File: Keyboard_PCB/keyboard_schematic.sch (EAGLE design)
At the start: 266 parts, among them IC1 LMV321M5, M2 KEYSWITCH-RGBSMDLED-ALPSMX-1U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, M3 KEYSWITCH-RGBSMDLED-ALPSMX-1U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, M4 KEYSWITCH-RGBSMDLED-ALPSMX-1U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, M5 KEYSWITCH-RGBSMDLED-ALPSMX-1U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, M6 KEYSWITCH-RGBSMDLED-ALPSMX-1U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, T1 BC846, Y2 CRYSTAL-GROUNDEDSMD-3.2X2.5

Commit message: Updated Schematics and boards
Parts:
- removed IC2: (no value), controller-micro_atmel_jd:AT90USB-QFN
- removed U$2: PCB_USB_CDS_1, USB_pcb_connectors:PCB_USB_CDS_1
- added IC3: (no value), controller-micro_atmel_jd:AT90USB-TQFP
- added J1: 1-2295018-2, 1-2295018-2:1-2295018-2
- T1: value BC846 -> (none); device transistor:BC846 -> transistor:-NPN-SOT23-EBC
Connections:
- removed net COL11: EQUAL2.P0, KP_9.P0, KP_ASTERISK.P0, KP_DASH.P0, NEXTSONG.P0, PAUSEPLAY.P0
- removed net ROW1.1: DF1.C, DF11.C, DF3.C, DF5.C, DF7.C, DF9.C, DM6.C, DNEXTSONG1.C, DPAUSE.C, DPAUSEPLAY.C, DSCROLLLOCK.C, DVOLUMEUP.C
- removed net ROW1.2: DBACKSONG.C, DESC.C, DF10.C, DF12.C, DF2.C, DF4.C, DF6.C, DF8.C, DLOCK.C, DNEXTSONG.C, DPRTSC.C, DVOLUMNEDOWN.C
- removed net ROW2.1: D1.C, D3.C, D5.C, D7.C, D9.C, DBACKSPACE.C, DDASH.C, DHOME.C, DKP_DASH.C, DKP_SLASH.C, DM5.C
- removed net ROW2.2: D0.C, D2.C, D4.C, D6.C, D8.C, DEQUAL.C, DGRAVE.C, DINSERT.C, DKP_ASTERISK.C, DNUMLOCK.C, DPGUP.C, DUNDERSCORE.C
- removed net ROW3.1: DBACKSLASH.C, DE.C, DEND.C, DEQUAL2.C, DKP_8.C, DLBRACKET.C, DM4.C, DO.C, DQ.C, DT.C, DU.C
- removed net ROW3.2: DDELETE.C, DI.C, DKP_5.C, DKP_7.C, DKP_9.C, DP.C, DPGDN.C, DR.C, DRBRACKET.C, DTAB.C, DW.C, DY.C
- removed net ROW4.1: DA.C, DCTRL2.C, DD.C, DG.C, DJ.C, DKP_4.C, DKP_6.C, DKP_62.C, DL.C, DM3.C, DQUOTE.C
- removed net ROW4.2: DCAPSLOCK.C, DENTER.C, DENTER2.C, DF.C, DH.C, DK.C, DKP_52.C, DS.C, DSEMICOLON.C, DUP.C
- removed net ROW5.1: DB.C, DC.C, DKP_2.C, DLEFT.C, DM.C, DM2.C, DMENU.C, DPERIOD.C, DZ.C
- removed net ROW5.2: DCOMMA.C, DDELETE2.C, DKP_1.C, DKP_3.C, DN.C, DRIGHT.C, DSHIFT.C, DSHIFT2.C, DSLASH.C, DV.C, DX.C
- removed net ROW6.1: DALT.C, DALT2.C, DBACKSPACE_1.C, DCTRL.C, DDOWN.C, DKP_0.C, DKP_DEL.C, DM1.C, DSPACE.C, DWIN.C, DWIN2.C
- new net COL13: 0.P0, F10.P0, P.P0, SEMICOLON.P0, SLASH.P0, WIN2.P0
- new net COL14: DASH.P0, F11.P0, LBRACKET.P0, MENU.P0, QUOTE.P0
- new net COL15: EQUAL.P0, F12.P0, RBRACKET.P0
- new net COL16: VOLUMEUP.P0
- new net COL17: BACKSLASH.P0, BACKSPACE.P0, CTRL2.P0, ENTER.P0, SHIFT2.P0, VOLUMNEDOWN.P0
- new net COL18: DELETE.P0, INSERT.P0, LEFT.P0, PRTSC.P0
- new net COL19: DOWN.P0, END.P0, HOME.P0, SCROLLLOCK.P0, UP.P0
- new net COL20: PAUSE.P0, PGDN.P0, PGUP.P0, RIGHT.P0
- new net COL21: BACKSONG.P0, KP_0.P0, KP_1.P0, KP_4.P0, KP_7.P0, NUMLOCK.P0
- new net COL22: KP_2.P0, KP_52.P0, KP_8.P0, KP_SLASH.P0, PAUSEPLAY.P0
- new net COL23: KP_3.P0, KP_6.P0, KP_9.P0, KP_ASTERISK.P0, KP_DEL.P0, NEXTSONG.P0
- new net COL24: ENTER2.P0, EQUAL2.P0, KP_DASH.P0, RANDSONG.P0
- new net COL25: BACKSPACE_1.P0, KP_5.P0, KP_62.P0, KP_DELETE2.P0, LOCK.P0, UNDERSCORE.P0
- new net LED1: M6.DI
- new net LED2: M5.DI
- new net LED3: M4.DI
- new net LED4: M3.DI
- new net LED5: M2.DI
- new net LED6: CTRL1.DI
- new net N$107: ESC.DI, M6.DO
- new net N$118: ESC.DO, F1.DI
- new net N$119: F1.DO, F2.DI
- new net N$121: F2.DO, F3.DI
- new net N$122: F3.DO, F4.DI
- new net N$123: F4.DO, F5.DI
- new net N$124: F5.DO, F6.DI
- new net N$132: F6.DO, F7.DI
- new net N$133: F7.DO, F8.DI
- new net N$134: F8.DO, F9.DI
- new net N$135: F10.DI, F9.DO
- new net N$136: F10.DO, F11.DI
- new net N$137: F11.DO, F12.DI
- new net N$138: F12.DO, VOLUMEUP.DI
- new net N$139: VOLUMEUP.DO, VOLUMNEDOWN.DI
- new net N$140: PRTSC.DI, VOLUMNEDOWN.DO
- new net N$141: PRTSC.DO, SCROLLLOCK.DI
- new net N$142: PAUSE.DI, SCROLLLOCK.DO
- new net N$143: BACKSONG.DI, PAUSE.DO
- new net N$144: BACKSONG.DO, PAUSEPLAY.DI
- new net N$145: NEXTSONG.DI, PAUSEPLAY.DO
- new net N$146: NEXTSONG.DO, RANDSONG.DI
- new net N$147: LOCK.DI, RANDSONG.DO
- new net N$148: IC3.PA1_AD1
- new net N$149: GRAVE.DI, M5.DO
- new net N$150: 1.DI, GRAVE.DO
- new net N$151: 1.DO, 2.DI
- new net N$152: 2.DO, 3.DI
- new net N$153: 3.DO, 4.DI
- new net N$154: 4.DO, 5.DI
- new net N$155: 5.DO, 6.DI
- new net N$156: 6.DO, 7.DI
- new net N$157: 7.DO, 8.DI
- new net N$158: 8.DO, 9.DI
- new net N$159: 0.DI, 9.DO
- new net N$160: 0.DO, DASH.DI
- new net N$161: DASH.DO, EQUAL.DI
- new net N$162: IC3.PA2_AD2
- new net N$163: BACKSPACE.DI, EQUAL.DO
- new net N$164: BACKSPACE.DO, INSERT.DI
- new net N$165: HOME.DI, INSERT.DO
- new net N$166: HOME.DO, PGUP.DI
- new net N$167: NUMLOCK.DI, PGUP.DO
- new net N$168: KP_SLASH.DI, NUMLOCK.DO
- new net N$169: KP_ASTERISK.DI, KP_SLASH.DO
- new net N$170: KP_ASTERISK.DO, KP_DASH.DI
- new net N$171: KP_DASH.DO, UNDERSCORE.DI
- new net N$172: M4.DO, TAB.DI
- new net N$173: Q.DI, TAB.DO
- new net N$174: Q.DO, W.DI
- new net N$175: E.DI, W.DO
- new net N$176: E.DO, R.DI
- new net N$177: R.DO, T.DI
- new net N$178: T.DO, Y.DI
- new net N$179: U.DI, Y.DO
- new net N$180: I.DI, U.DO
- new net N$181: I.DO, O.DI
- new net N$182: O.DO, P.DI
- new net N$183: LBRACKET.DI, P.DO
- new net N$184: LBRACKET.DO, RBRACKET.DI
- new net N$185: BACKSLASH.DI, RBRACKET.DO
- new net N$186: IC3.PA3_AD3
- new net N$187: BACKSLASH.DO, DELETE.DI
- new net N$188: DELETE.DO, END.DI
- new net N$189: END.DO, PGDN.DI
- new net N$190: KP_7.DI, PGDN.DO
- new net N$191: KP_7.DO, KP_8.DI
- new net N$192: KP_8.DO, KP_9.DI
- new net N$193: EQUAL2.DI, KP_9.DO
- new net N$194: EQUAL2.DO, KP_5.DI
- new net N$195: CAPSLOCK.DI, M3.DO
- new net N$196: A.DI, CAPSLOCK.DO
- new net N$197: A.DO, S.DI
- new net N$198: D.DI, S.DO
- new net N$199: D.DO, F.DI
- new net N$200: F.DO, G.DI
- new net N$201: G.DO, H.DI
- new net N$202: H.DO, J.DI
- new net N$203: J.DO, K.DI
- new net N$204: K.DO, L.DI
- new net N$205: L.DO, SEMICOLON.DI
- new net N$206: QUOTE.DI, SEMICOLON.DO
- new net N$207: ENTER.DI, QUOTE.DO
- new net N$208: ENTER.DO, KP_4.DI
- new net N$209: ENTER2.DI, KP_3.DO
- new net N$210: KP_4.DO, KP_52.DI
- new net N$211: KP_52.DO, KP_6.DI
- new net N$212: KP_6.DO, KP_62.DI
- new net N$213: IC3.PA4_AD4
- new net N$214: M2.DO, SHIFT.DI
- new net N$215: SHIFT.DO, Z.DI
- new net N$216: X.DI, Z.DO
- new net N$217: C.DI, X.DO
- new net N$218: C.DO, V.DI
- new net N$219: B.DI, V.DO
- new net N$220: B.DO, N.DI
- new net N$221: M.DI, N.DO
- new net N$222: COMMA.DI, M.DO
- new net N$223: COMMA.DO, PERIOD.DI
- new net N$224: PERIOD.DO, SLASH.DI
- new net N$225: SHIFT2.DI, SLASH.DO
- new net N$226: IC3.PA5_AD5
- new net N$227: KP_1.DO, KP_2.DI
- new net N$228: KP_2.DO, KP_3.DI
- new net N$229: ENTER2.DO, KP_DELETE2.DI
- new net N$230: KP_1.DI, SHIFT2.DO
- new net N$231: IC3.PA6_AD6
- new net N$232: CTRL.DI, CTRL1.DO
- new net N$233: CTRL.DO, WIN.DI
- new net N$234: ALT.DI, WIN.DO
- new net N$235: ALT.DO, SPACE.DI
- new net N$236: IC3.PA7_AD7
- new net N$238: ALT2.DI, SPACE.DO
- new net N$239: J1.VBUS@4
- new net N$242: ALT2.DO, WIN2.DI
- new net N$243: MENU.DI, WIN2.DO
- new net N$245: CTRL2.DI, MENU.DO
- new net N$246: CTRL2.DO, LEFT.DI
- new net N$247: KP_0.DI
- new net N$248: KP_0.DO, KP_DEL.DI
- new net N$249: BACKSPACE_1.DI, KP_DEL.DO
- new net N$250: DOWN.DI, LEFT.DO
- new net N$251: DOWN.DO, RIGHT.DI
- new net N$252: RIGHT.DO
- new net ROW1: DBACKSONG.C, DESC.C, DF1.C, DF10.C, DF11.C, DF12.C, DF2.C, DF3.C, DF4.C, DF5.C, DF6.C, DF7.C, DF8.C, DF9.C, DLOCK.C, DM6.C, DNEXTSONG.C, DNEXTSONG1.C, DPAUSE.C, DPAUSEPLAY.C, DPRTSC.C, DSCROLLLOCK.C, DVOLUMEUP.C, DVOLUMNEDOWN.C
- new net ROW2: D0.C, D1.C, D2.C, D3.C, D4.C, D5.C, D6.C, D7.C, D8.C, D9.C, DBACKSPACE.C, DDASH.C, DEQUAL.C, DGRAVE.C, DHOME.C, DINSERT.C, DKP_ASTERISK.C, DKP_DASH.C, DKP_SLASH.C, DM5.C, DNUMLOCK.C, DPGUP.C, DUNDERSCORE.C
- new net ROW3: DBACKSLASH.C, DDELETE.C, DE.C, DEND.C, DEQUAL2.C, DI.C, DKP_5.C, DKP_7.C, DKP_8.C, DKP_9.C, DLBRACKET.C, DM4.C, DO.C, DP.C, DPGDN.C, DQ.C, DR.C, DRBRACKET.C, DT.C, DTAB.C, DU.C, DW.C, DY.C
- new net ROW4: DA.C, DCAPSLOCK.C, DD.C, DENTER.C, DF.C, DG.C, DH.C, DJ.C, DK.C, DKP_4.C, DKP_52.C, DKP_6.C, DKP_62.C, DL.C, DM3.C, DQUOTE.C, DS.C, DSEMICOLON.C
- new net ROW5: DB.C, DC.C, DCOMMA.C, DDELETE2.C, DENTER2.C, DKP_1.C, DKP_2.C, DKP_3.C, DM.C, DM2.C, DN.C, DPERIOD.C, DSHIFT.C, DSHIFT2.C, DSLASH.C, DUP.C, DV.C, DX.C, DZ.C
- new net ROW6: DALT.C, DALT2.C, DBACKSPACE_1.C, DCTRL2.C, DDOWN.C, DKP_0.C, DKP_DEL.C, DLEFT.C, DM1.C, DMENU.C, DRIGHT.C, DSPACE.C, DWIN.C, DWIN2.C
- net +5V: now also IC3.AREF, IC3.AVCC, IC3.VCC, IC3.VCC@1, J1.VBUS@1, J1.VBUS@2, J1.VBUS@3; no longer IC2.AREF, IC2.AVCC, IC2.VCC, IC2.VCC@1, U$2.A4, U$2.A9, U$2.B4, U$2.B9
- net CC1: now also IC1.+IN, J1.CC1, R6.2; no longer R5.1, U$2.A5
- net CC2: now also J1.CC2, R5.1; no longer IC1.+IN, R6.2, U$2.B5
- net COL1: no longer CAPSLOCK.P0, ESC.P0, GRAVE.P0, SHIFT.P0, TAB.P0
- net COL10: now also 8.P0, COMMA.P0, F8.P0, I.P0, K.P0; no longer BACKSONG.P0, ENTER2.P0, KP_3.P0, KP_6.P0, KP_7.P0, KP_8.P0, KP_DEL.P0, KP_SLASH.P0, NUMLOCK.P0, PAUSE.P0
- net COL12: now also 9.P0, ALT2.P0, F9.P0, L.P0, O.P0, PERIOD.P0; no longer BACKSPACE_1.P0, KP_5.P0, KP_62.P0, KP_DELETE2.P0, LOCK.P0, RANDSONG.P0, UNDERSCORE.P0
- net COL2: now also CAPSLOCK.P0, ESC.P0, GRAVE.P0, SHIFT.P0, TAB.P0; no longer 1.P0, 2.P0, A.P0, F1.P0, F2.P0, Q.P0, S.P0, W.P0, X.P0, Z.P0
- net COL3: now also 1.P0, A.P0, F1.P0, Q.P0, Z.P0; no longer 3.P0, 4.P0, C.P0, D.P0, E.P0, F.P0, F3.P0, F4.P0, R.P0, V.P0
- net COL4: now also 2.P0, F2.P0, S.P0, W.P0, X.P0; no longer 5.P0, 6.P0, B.P0, F5.P0, F6.P0, G.P0, H.P0, N.P0, T.P0, Y.P0
- net COL5: now also 3.P0, C.P0, D.P0, E.P0, F3.P0; no longer 7.P0, 8.P0, COMMA.P0, F7.P0, F8.P0, I.P0, J.P0, K.P0, M.P0, SPACE.P0, U.P0
- net COL6: now also 4.P0, F.P0, F4.P0, R.P0, V.P0; no longer 0.P0, 9.P0, ALT2.P0, F10.P0, F9.P0, L.P0, O.P0, P.P0, PERIOD.P0, SEMICOLON.P0, SLASH.P0
- net COL7: now also 5.P0, B.P0, F5.P0, G.P0, SPACE.P0, T.P0; no longer DASH.P0, ENTER.P0, EQUAL.P0, F11.P0, F12.P0, LBRACKET.P0, MENU.P0, QUOTE.P0, RBRACKET.P0, SHIFT2.P0, WIN2.P0
- net COL8: now also 6.P0, F6.P0, H.P0, N.P0, Y.P0; no longer BACKSLASH.P0, BACKSPACE.P0, CTRL2.P0, DELETE.P0, DOWN.P0, INSERT.P0, LEFT.P0, RIGHT.P0, UP.P0, VOLUMEUP.P0, VOLUMNEDOWN.P0
- net COL9: now also 7.P0, F7.P0, J.P0, M.P0, U.P0; no longer END.P0, HOME.P0, KP_0.P0, KP_1.P0, KP_2.P0, KP_4.P0, KP_52.P0, PGDN.P0, PGUP.P0, PRTSC.P0, SCROLLLOCK.P0
- net D+32U: now also IC3.D+; no longer IC2.D+
- net D+USB: now also J1.D+@1; no longer U$2.A6
- net D-32U4: now also IC3.D-; no longer IC2.D-
- net D-USB: now also J1.D-@1; no longer U$2.A7
- net GND: now also IC3.AGND, IC3.GND, IC3.GND@1, IC3.UGND, J1.GND@1, J1.GND@2, J1.GND@3, J1.GND@4, J1.SHIELD; no longer IC2.AGND, IC2.GND, IC2.GND@1, IC2.UGND, U$2.A1, U$2.A12, U$2.B1, U$2.B12
- net N$102: now also IC3.PA0_AD0; no longer CTRL.P1, DCTRL.A
- net PE2: now also IC3.PE2_ALE_HWB; no longer IC2.PE2_ALE_HWB
- net RESET: now also IC3./RESET; no longer IC2./RESET
- net UCAP: now also IC3.UCAP; no longer IC2.UCAP
- net XTAL1: now also IC3.XTAL1; no longer IC2.XTAL1
- net XTAL2: now also IC3.XTAL2; no longer IC2.XTAL2
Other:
- moved on the sheet: 1, A, ALT, ALT2, B, BACKSLASH, BACKSPACE, C, COMMA, CTRL2, D, D0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

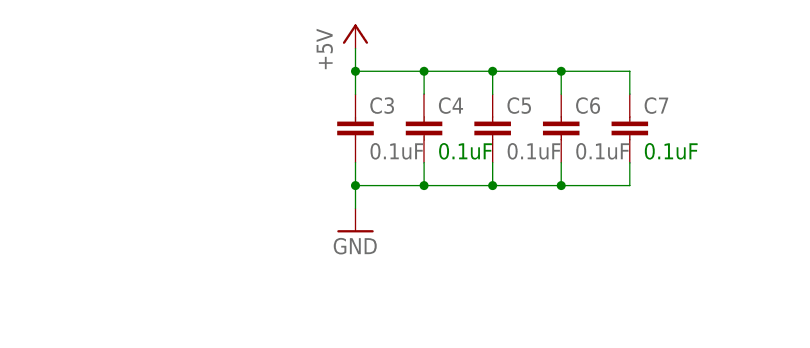
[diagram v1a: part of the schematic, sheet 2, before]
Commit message: Updated board
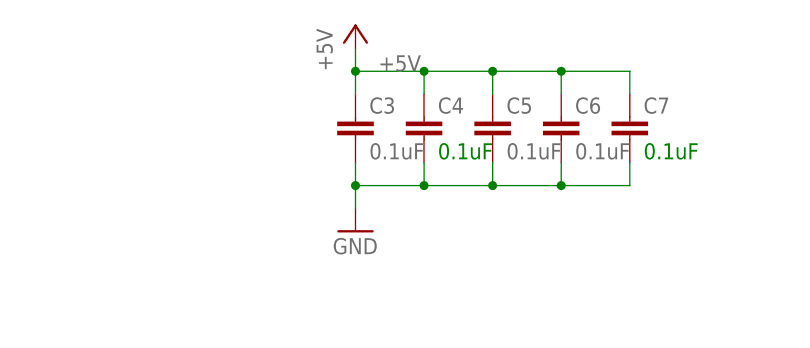
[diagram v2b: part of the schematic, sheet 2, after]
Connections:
- net +5V: now also C3.1, C4.1, C5.1, C6.1, C7.1
- net VCC: no longer C3.1, C4.1, C5.1, C6.1, C7.1
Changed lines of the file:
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@@
 <net name="VCC" class="0">
-<segment>
-<pinref part="C3" gate="G$1" pin="1"/>
-<wire x1="-137.16" y1="154.94" x2="-137.16" y2="157.48" width="0.1524" layer="91"/>
-<wire x1="-137.16" y1="157.48" x2="-129.54" y2="157.48" width="0.1524" layer="91"/>
-<pinref part="C7" gate="G$1" pin="1"/>
-<wire x1="-129.54" y1="157.48" x2="-121.92" y2="157.48" width="0.1524" layer="91"/>
-<wire x1="-121.92" y1="157.48" x2="-114.3" y2="157.48" width="0.1524" layer="91"/>
-<wire x1="-114.3" y1="157.48" x2="-106.68" y2="157.48" width="0.1524" layer="91"/>
-<wire x1="-106.68" y1="157.48" x2="-106.68" y2="154.94" width="0.1524" layer="91"/>
-<pinref part="C6" gate="G$1" pin="1"/>
-<wire x1="-114.3" y1="154.94" x2="-114.3" y2="157.48" width="0.1524" layer="91"/>
-<junction x="-114.3" y="157.48"/>
-<pinref part="C5" gate="G$1" pin="1"/>
-<wire x1="-121.92" y1="154.94" x2="-121.92" y2="157.48" width="0.1524" layer="91"/>
-<junction x="-121.92" y="157.48"/>
-<pinref part="C4" gate="G$1" pin="1"/>
-<wire x1="-129.54" y1="154.94" x2="-129.54" y2="157.48" width="0.1524" layer="91"/>
-<junction x="-129.54" y="157.48"/>
-<wire x1="-137.16" y1="157.48" x2="-137.16" y2="160.02" width="0.1524" layer="91"/>
-<junction x="-137.16" y="157.48"/>
-<pinref part="P+1" gate="1" pin="+5V"/>
-</segment>
 <segment>
 <pinref part="P+2" gate="1" pin="+5V"/>
@@
 <pinref part="P+7" gate="1" pin="+5V"/>
 </segment>
+<segment>
+<pinref part="C3" gate="G$1" pin="1"/>
+<wire x1="-137.16" y1="154.94" x2="-137.16" y2="157.48" width="0.1524" layer="91"/>
+<wire x1="-137.16" y1="157.48" x2="-129.54" y2="157.48" width="0.1524" layer="91"/>
+<pinref part="C7" gate="G$1" pin="1"/>
+<wire x1="-129.54" y1="157.48" x2="-121.92" y2="157.48" width="0.1524" layer="91"/>
+<wire x1="-121.92" y1="157.48" x2="-114.3" y2="157.48" width="0.1524" layer="91"/>
+<wire x1="-114.3" y1="157.48" x2="-106.68" y2="157.48" width="0.1524" layer="91"/>
+<wire x1="-106.68" y1="157.48" x2="-106.68" y2="154.94" width="0.1524" layer="91"/>
+<pinref part="C6" gate="G$1" pin="1"/>
+<wire x1="-114.3" y1="154.94" x2="-114.3" y2="157.48" width="0.1524" layer="91"/>
+<junction x="-114.3" y="157.48"/>
+<pinref part="C5" gate="G$1" pin="1"/>
+<wire x1="-121.92" y1="154.94" x2="-121.92" y2="157.48" width="0.1524" layer="91"/>
+<junction x="-121.92" y="157.48"/>
+<pinref part="C4" gate="G$1" pin="1"/>
+<wire x1="-129.54" y1="154.94" x2="-129.54" y2="157.48" width="0.1524" layer="91"/>
+<junction x="-129.54" y="157.48"/>
+<wire x1="-137.16" y1="157.48" x2="-137.16" y2="160.02" width="0.1524" layer="91"/>
+<junction x="-137.16" y="157.48"/>
+<pinref part="P+1" gate="1" pin="+5V"/>
+<label x="-134.62" y="157.48" size="1.778" layer="95"/>
+</segment>
 </net>

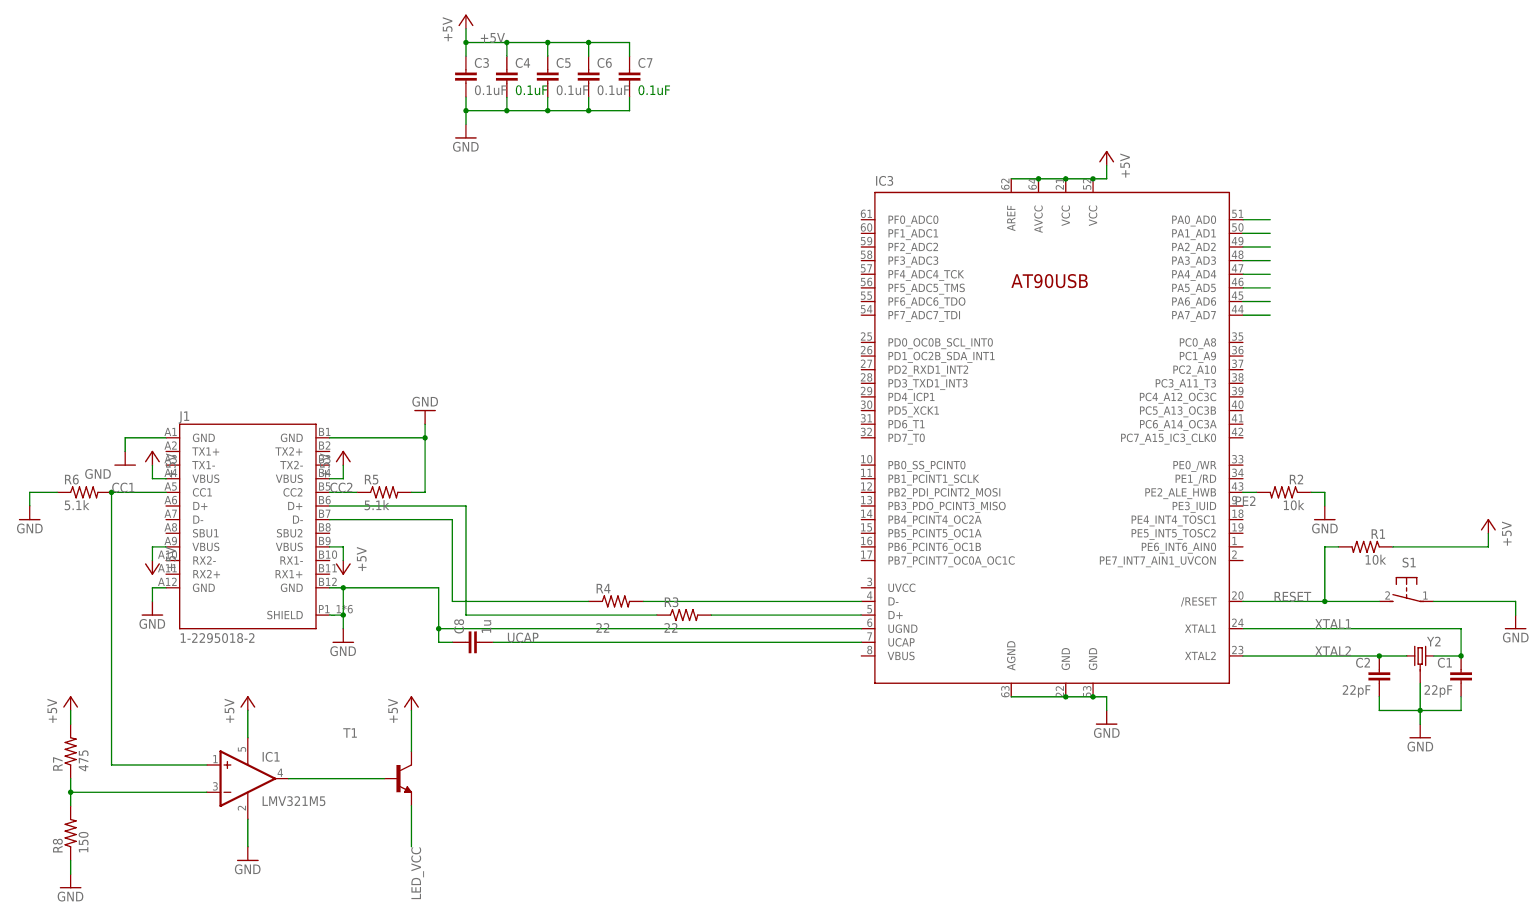
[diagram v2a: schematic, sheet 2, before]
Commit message: Updated Board
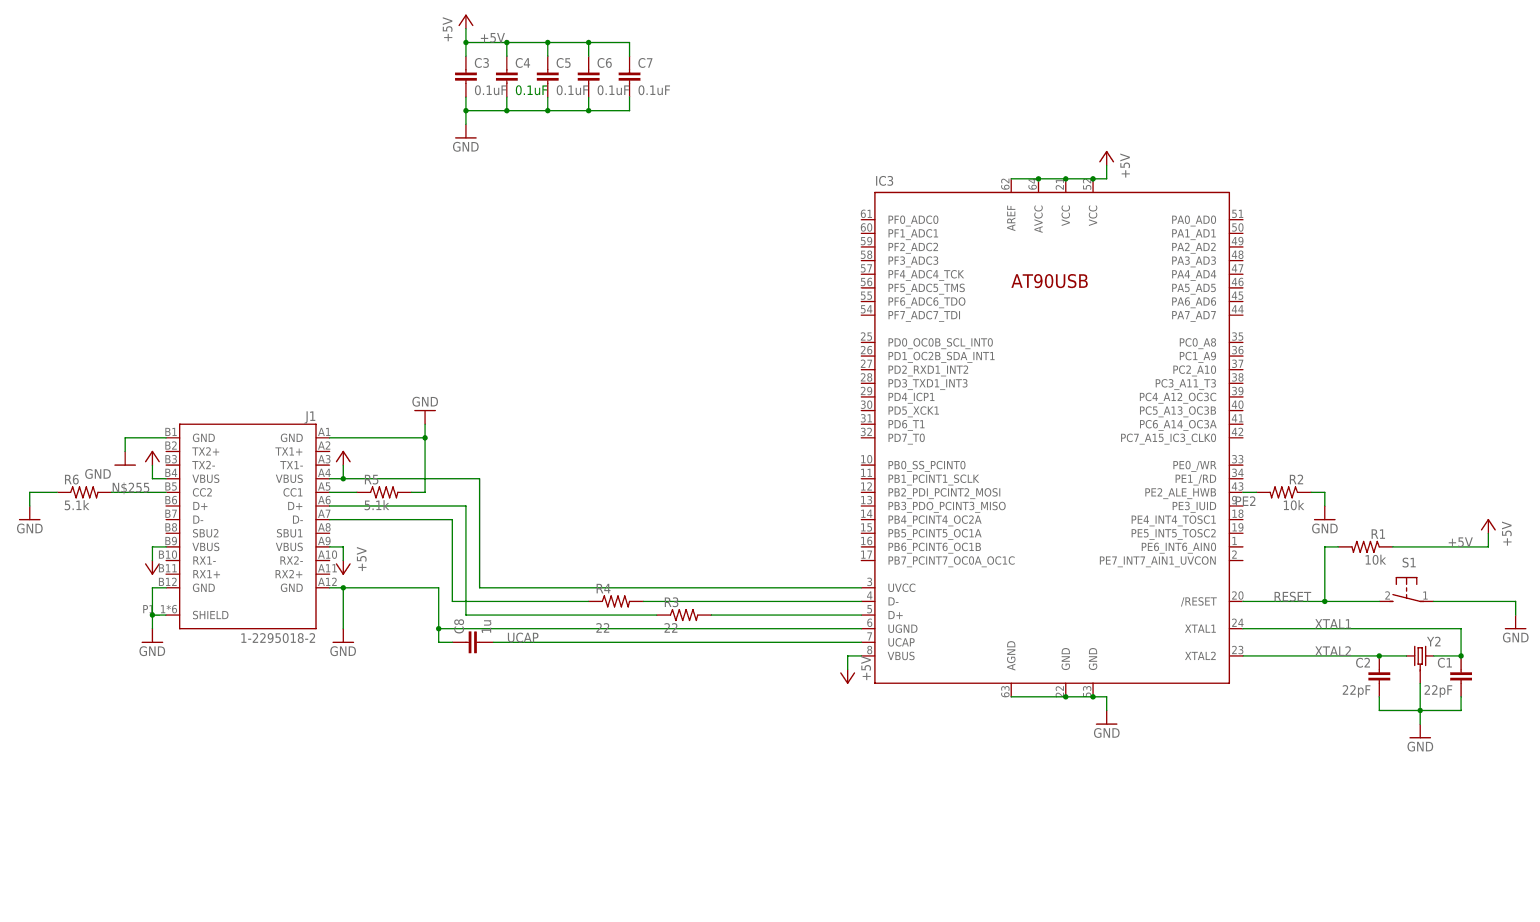
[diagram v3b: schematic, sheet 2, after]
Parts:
- removed IC1: LMV321M5, linear:LMV321M5
- removed R7: 475, rcl:R-US_M0805
- removed R8: 150, rcl:R-US_M0805
- removed T1: (no value), transistor:-NPN-SOT23-EBC
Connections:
- removed net CC1: IC1.+IN, J1.CC1, R6.2
- removed net CC2: J1.CC2, R5.1
- removed net LED_VCC: T1.E
- removed net N$102: IC3.PA0_AD0
- removed net N$116: IC1.-IN, R7.1, R8.2
- removed net N$117: IC1.OUT, T1.B
- removed net N$148: IC3.PA1_AD1
- removed net N$162: IC3.PA2_AD2
- removed net N$186: IC3.PA3_AD3
- removed net N$213: IC3.PA4_AD4
- removed net N$226: IC3.PA5_AD5
- removed net N$231: IC3.PA6_AD6
- removed net N$236: IC3.PA7_AD7
- removed net VCC: R1.1
- new net N$237: J1.CC1, R5.1
- new net N$255: J1.CC2, R6.2
- net +5V: now also IC3.UVCC, IC3.VBUS, J1.VBUS@4, R1.1; no longer IC1.V+, J1.VBUS@2, R7.2, T1.C
- net D+USB: now also J1.D+; no longer J1.D+@1
- net D-USB: now also J1.D-; no longer J1.D-@1
- net GND: no longer IC1.V-, R8.1
- net N$239: now also J1.VBUS@2; no longer J1.VBUS@4
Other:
- moved on the sheet: J1
